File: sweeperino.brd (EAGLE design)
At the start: 100 x 79.9 mm, 41 parts, among them IC2 Si570, IC3 LM1117-3.3V, IC5 7805TV, IC6 7805TV, M1 ARDUINO-NANO-3.0, U1 AD8307ARZ, X1 VFO, X2 VFO

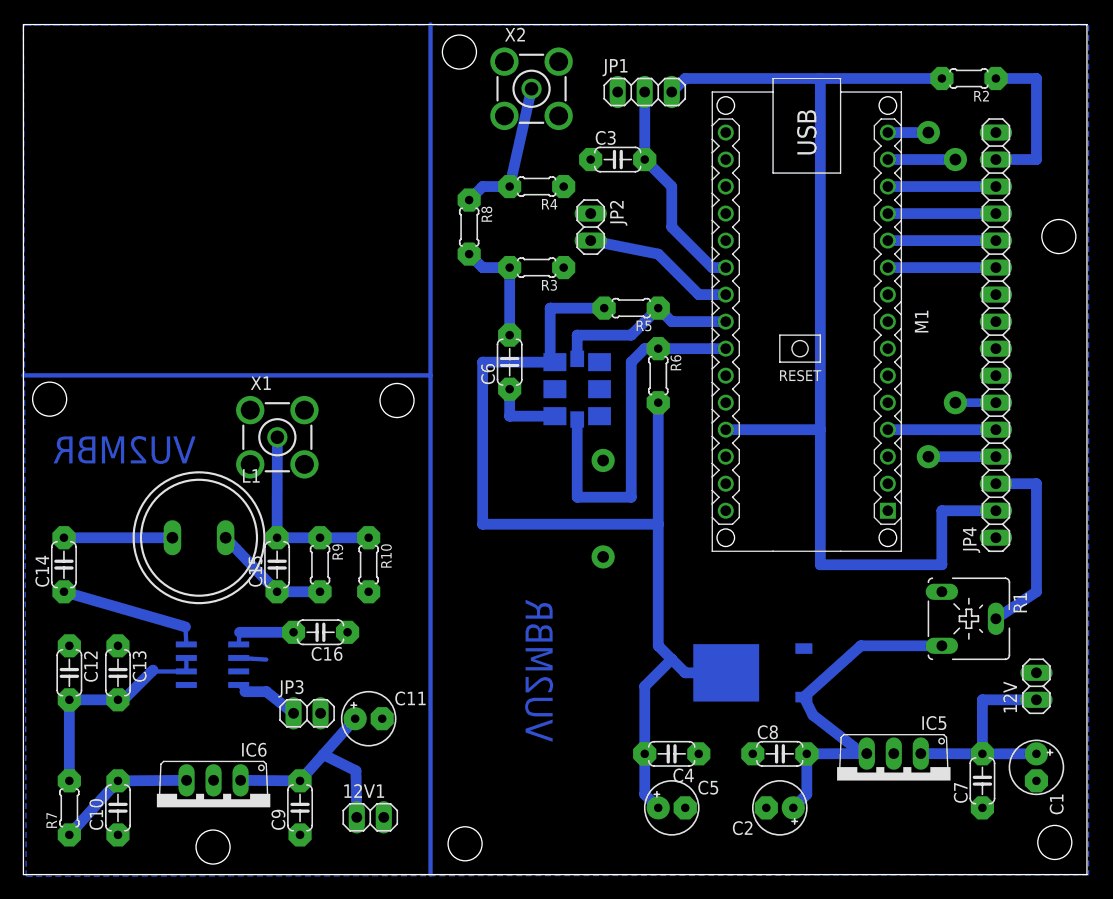
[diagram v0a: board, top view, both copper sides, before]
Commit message: Updated board
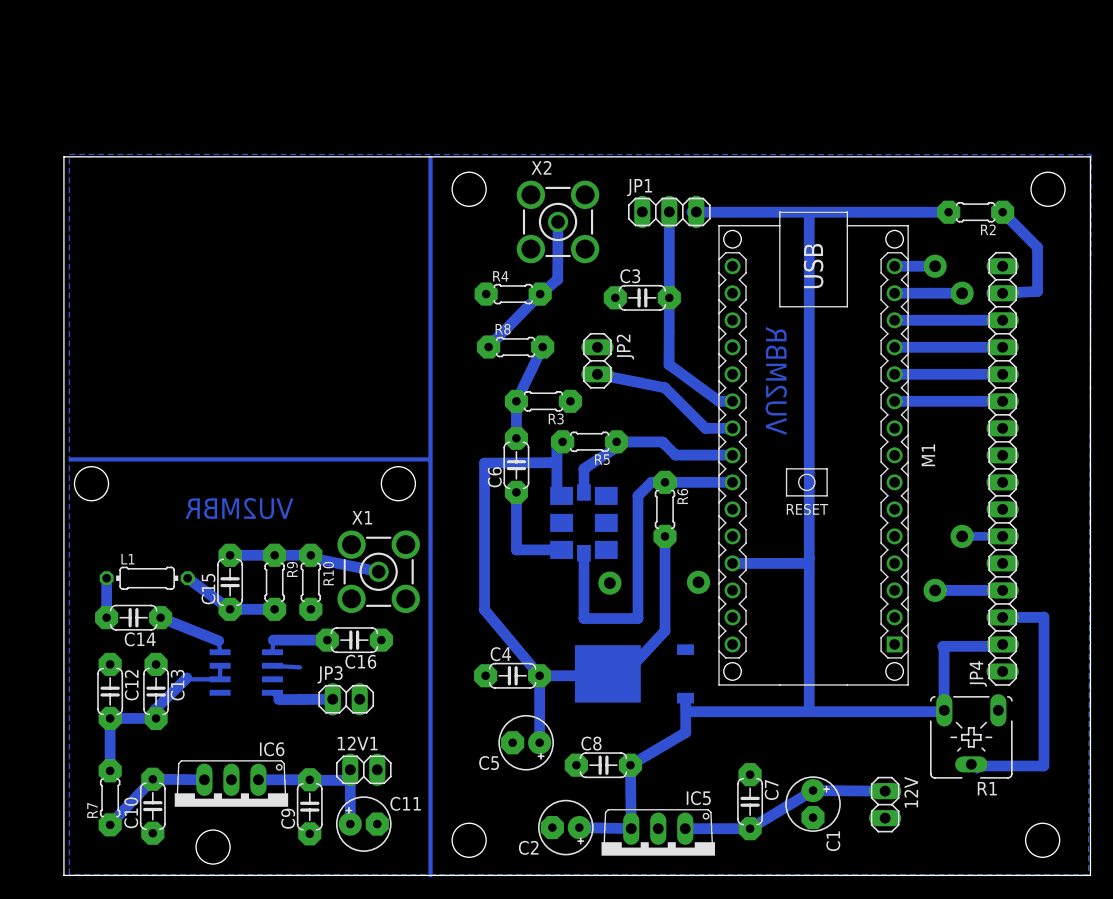
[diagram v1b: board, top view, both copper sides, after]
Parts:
- L1: device inductor-neosid:SD12_1000 -> eagle-ltspice:0204/7
- moved IC5 23.2 mm to (59.7, 4.39)
- moved C7 21.9 mm to (68.3, 9.47), turned to 270 degrees
- moved C1 21.3 mm to (74.2, 9.25)
- moved C2 20.2 mm to (51.0, 7.04)
- moved 12V 18.1 mm to (81.0, 9.19), turned to 270 degrees
- moved C4 16.7 mm to (46.0, 21.3), turned to 0 degrees
- moved C8 16.6 mm to (54.5, 12.9)
- moved X1 15.8 mm to (33.4, 31.1)
- moved C5 15.0 mm to (47.3, 15.0), turned to 180 degrees
- moved C3 13.2 mm to (58.2, 56.8)
- moved R5 13.2 mm to (53.2, 43.3)
- moved X2 12.8 mm to (50.3, 64.0)
- moved IC2 12.6 mm to (52.7, 35.7)
- moved JP2 12.6 mm to (54.0, 50.9)
- moved JP4 12.6 mm to (92.1, 40.8)
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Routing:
- net N$21: track 94.6 -> 68.9 mm
- net N$27: track 79.9 -> 67.4 mm
- net GND: track 11.5 -> 2.60 mm
- net N$5: track 17.3 -> 24.4 mm
- net N$15: track 21.2 -> 14.5 mm
- net N$3: track 13.6 -> 6.96 mm
- net N$18: track 10.2 -> 3.71 mm
- net N$19: track 17.8 -> 22.5 mm
- net N$28: track 38.3 -> 33.7 mm
- net N$25: track 18.1 -> 14.8 mm
- net N$22: track 6.79 -> 9.66 mm
- net N$2: track 13.3 -> 10.7 mm
- net N$16: track 21.4 -> 18.9 mm
- net N$20: track 34.5 -> 32.2 mm
- net N$23: track 11.1 -> 9.13 mm
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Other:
- board size 100 x 79.9 mm -> 96.5 x 67.6 mm
